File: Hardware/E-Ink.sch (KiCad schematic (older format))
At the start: 4 parts

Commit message: safe commit
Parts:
- removed J?: Micro_USB, digikey-footprints:USB_Micro_B_Female_1050170001, symbol E-Ink:Micro_USB
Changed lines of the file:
@@
 EESchema Schematic File Version 4
-LIBS:E-Ink-cache
 EELAYER 30 0
 EELAYER END
@@
 	1    0    0    -1
 $EndComp
-$Comp
-L E-Ink:Micro_USB J?
-U 1 1 5DC9DD54
-P 4850 2000
-F 0 "J?" H 4914 2723 50  0000 C CNN
-F 1 "Micro_USB" H 4914 2632 50  0000 C CNN
-F 2 "digikey-footprints:USB_Micro_B_Female_1050170001" H 5050 2200 60  0001 L CNN
-F 3 "https://www.molex.com/pdm_docs/sd/1050170001_sd.pdf" H 5050 2300 60  0001 L CNN
-F 4 "WM1399CT-ND" H 5050 2400 60  0001 L CNN "Digi-Key_PN"
-F 5 "1050170001" H 5050 2500 60  0001 L CNN "MPN"
-F 6 "Connectors, Interconnects" H 5050 2600 60  0001 L CNN "Category"
-F 7 "USB, DVI, HDMI Connectors" H 5050 2700 60  0001 L CNN "Family"
-F 8 "https://www.molex.com/pdm_docs/sd/1050170001_sd.pdf" H 5050 2800 60  0001 L CNN "DK_Datasheet_Link"
-F 9 "/product-detail/en/molex/1050170001/WM1399CT-ND/2350885" H 5050 2900 60  0001 L CNN "DK_Detail_Page"
-F 10 "CONN RCPT USB2.0 MICRO B SMD R/A" H 5050 3000 60  0001 L CNN "Description"
-F 11 "Molex" H 5050 3100 60  0001 L CNN "Manufacturer"
-F 12 "Active" H 5050 3200 60  0001 L CNN "Status"
-	1    4850 2000
-	1    0    0    -1
-$EndComp

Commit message: Save commit after work at OTH
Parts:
- removed U?: LDO-3.3V, E-Ink:WSON-6-1EP_3x3mm_P0.95mm, symbol E-Ink:LDO-3.3V
- removed U?: LDO-5.0V, E-Ink:WSON-6-1EP_3x3mm_P0.95mm, symbol E-Ink:LDO-5.0V
- added J?: S8B-PH-SM4-TB, symbol E-Ink:S8B-PH-SM4-TB
- added U?: TXB0104PWR, digikey-footprints:TSSOP-14_W4.4mm, symbol E-Ink:TXB0104PWR
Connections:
- net labels added: +3V3, +5V, BSY_IT8951, CS, EN_SPI, GND, MISO, MOSI, RST_8951, SCK
- wire segments 0 -> 8
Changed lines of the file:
@@
 EESchema Schematic File Version 4
-EELAYER 30 0
+LIBS:E-Ink-cache
+EELAYER 29 0
 EELAYER END
 $Descr A4 11693 8268
@@
 $EndComp
 $Comp
-L E-Ink:LDO-3.3V U?
-U 1 1 5DCA3BF6
-P 4850 3850
-F 0 "U?" H 4925 4555 50  0000 C CNN
-F 1 "LDO-3.3V" H 4925 4464 50  0000 C CNN
-F 2 "E-Ink:WSON-6-1EP_3x3mm_P0.95mm" H 5100 3750 50  0001 C CNN
-F 3 "http://www.ti.com/general/docs/suppproductinfo.tsp?distId=10&gotoUrl=http%3A%2F%2Fwww.ti.com%2Flit%2Fgpn%2Flp38690" H 4700 4450 50  0001 C CNN
-F 4 "LP38692SD-3.3/NOPBCT-ND" H 4925 4373 50  0000 C CNN "Digi-Key_PN"
-	1    4850 3850
+L E-Ink:S8B-PH-SM4-TB J?
+U 1 1 5DD86C25
+P 7100 1500
+F 0 "J?" H 7528 1201 50  0000 L CNN
+F 1 "S8B-PH-SM4-TB" H 7528 1110 50  0000 L CNN
+F 2 "" H 7050 1700 50  0001 C CNN
+F 3 "http://www.jst-mfg.com/product/pdf/eng/ePH.pdf" H 7050 1700 50  0001 C CNN
+F 4 "455-1755-1-ND" H 7450 1600 50  0001 C CNN "Digi-Key_PN"
+	1    7100 1500
 	1    0    0    -1
 $EndComp
 $Comp
-L E-Ink:LDO-5.0V U?
-U 1 1 5DCA47AE
-P 4950 4700
-F 0 "U?" H 4900 5305 50  0000 C CNN
-F 1 "LDO-5.0V" H 4900 5214 50  0000 C CNN
-F 2 "E-Ink:WSON-6-1EP_3x3mm_P0.95mm" H 5000 4500 50  0001 C CNN
-F 3 "http://www.ti.com/general/docs/suppproductinfo.tsp?distId=10&gotoUrl=http%3A%2F%2Fwww.ti.com%2Flit%2Fgpn%2Flp38690" H 4700 5200 50  0001 C CNN
-F 4 "LP38692SD-5.0/NOPBCT-ND" H 4900 5123 50  0000 C CNN "Digi-Key_PN"
-	1    4950 4700
+L power:GND #PWR?
+U 1 1 5DD8AF59
+P 2000 4200
+F 0 "#PWR?" H 2000 3950 50  0001 C CNN
+F 1 "GND" H 2005 4027 50  0000 C CNN
+F 2 "" H 2000 4200 50  0001 C CNN
+F 3 "" H 2000 4200 50  0001 C CNN
+	1    2000 4200
 	1    0    0    -1
 $EndComp
+$Comp
+L power:GND #PWR?
+U 1 1 5DD8BEF7
+P 7100 1600
+F 0 "#PWR?" H 7100 1350 50  0001 C CNN
+F 1 "GND" H 7105 1427 50  0000 C CNN
+F 2 "" H 7100 1600 50  0001 C CNN
+F 3 "" H 7100 1600 50  0001 C CNN
+	1    7100 1600
+	0    1    1    0
+$EndComp
+$Comp
+L power:+5V #PWR?
+U 1 1 5DD8C3B3
+P 7100 1500
+F 0 "#PWR?" H 7100 1350 50  0001 C CNN
+F 1 "+5V" H 7115 1673 50  0000 C CNN
+F 2 "" H 7100 1500 50  0001 C CNN
+F 3 "" H 7100 1500 50  0001 C CNN
+	1    7100 1500
+	1    0    0    -1
+$EndComp
+$Comp
+L power:+5V #PWR?
+U 1 1 5DD8E1F6
+P 4950 1350
+F 0 "#PWR?" H 4950 1200 50  0001 C CNN
+F 1 "+5V" H 4965 1523 50  0000 C CNN
+F 2 "" H 4950 1350 50  0001 C CNN
+F 3 "" H 4950 1350 50  0001 C CNN
+	1    4950 1350
+	1    0    0    -1
+$EndComp
+$Comp
+L power:+3V3 #PWR?
+U 1 1 5DD8E341
+P 4650 1350
+F 0 "#PWR?" H 4650 1200 50  0001 C CNN
+F 1 "+3V3" H 4665 1523 50  0000 C CNN
+F 2 "" H 4650 1350 50  0001 C CNN
+F 3 "" H 4650 1350 50  0001 C CNN
+	1    4650 1350
+	1    0    0    -1
+$EndComp
+Wire Wire Line
+	4650 1350 4750 1350
+Wire Wire Line
+	4750 1350 4750 1400
+Wire Wire Line
+	4850 1400 4850 1350
+Wire Wire Line
+	4850 1350 4950 1350
+$Comp
+L power:GND #PWR?
+U 1 1 5DD8FB9C
+P 4850 2400
+F 0 "#PWR?" H 4850 2150 50  0001 C CNN
+F 1 "GND" H 4855 2227 50  0000 C CNN
+F 2 "" H 4850 2400 50  0001 C CNN
+F 3 "" H 4850 2400 50  0001 C CNN
+	1    4850 2400
+	0    -1   -1   0
+$EndComp
+Wire Wire Line
+	5150 1700 7100 1700
+Wire Wire Line
+	7100 1800 5150 1800
+Wire Wire Line
+	5150 1900 7100 1900
+Wire Wire Line
+	7100 2000 5150 2000
+Text GLabel 4450 1700 0    50   Input ~ 0
+MISO
+Text GLabel 4450 1800 0    50   Input ~ 0
+MOSI
+Text GLabel 4450 1900 0    50   Input ~ 0
+SCK
+Text GLabel 4450 2000 0    50   Input ~ 0
+CS
+Text GLabel 4450 2100 0    50   Input ~ 0
+EN_SPI
+Text GLabel 7100 2100 0    50   Input ~ 0
+RST_8951
+Text GLabel 7100 2200 0    50   Input ~ 0
+BSY_IT8951
+Text GLabel 2600 2200 2    50   Input ~ 0
+MISO
+Text GLabel 2600 2300 2    50   Input ~ 0
+MOSI
+Text GLabel 2600 2400 2    50   Input ~ 0
+SCK
+Text GLabel 2600 2500 2    50   Input ~ 0
+CS
+$Comp
+L E-Ink:TXB0104PWR U?
+U 1 1 5DD8930F
+P 4850 1900
+F 0 "U?" H 4800 1303 60  0000 C CNN
+F 1 "TXB0104PWR" H 4921 1197 60  0000 C CNN
+F 2 "digikey-footprints:TSSOP-14_W4.4mm" H 5050 2100 60  0001 L CNN
+F 3 "http://www.ti.com/general/docs/suppproductinfo.tsp?distId=10&gotoUrl=http%3A%2F%2Fwww.ti.com%2Flit%2Fgpn%2Ftxb0104" H 5050 2200 60  0001 L CNN
+F 4 "296-21929-1-ND" H 5050 2300 60  0001 L CNN "Digi-Key_PN"
+F 5 "TXB0104PWR" H 5050 2400 60  0001 L CNN "MPN"
+F 6 "Integrated Circuits (ICs)" H 5050 2500 60  0001 L CNN "Category"
+F 7 "Logic - Translators, Level Shifters" H 5050 2600 60  0001 L CNN "Family"
+F 8 "http://www.ti.com/general/docs/suppproductinfo.tsp?distId=10&gotoUrl=http%3A%2F%2Fwww.ti.com%2Flit%2Fgpn%2Ftxb0104" H 5050 2700 60  0001 L CNN "DK_Datasheet_Link"
+F 9 "/product-detail/en/texas-instruments/TXB0104PWR/296-21929-1-ND/1629282" H 5050 2800 60  0001 L CNN "DK_Detail_Page"
+F 10 "IC TRNSLTR BIDIRECTIONAL 14TSSOP" H 5050 2900 60  0001 L CNN "Description"
+F 11 "Texas Instruments" H 5050 3000 60  0001 L CNN "Manufacturer"
+F 12 "Active" H 5050 3100 60  0001 L CNN "Status"
+	1    4850 1900
+	1    0    0    -1
+$EndComp

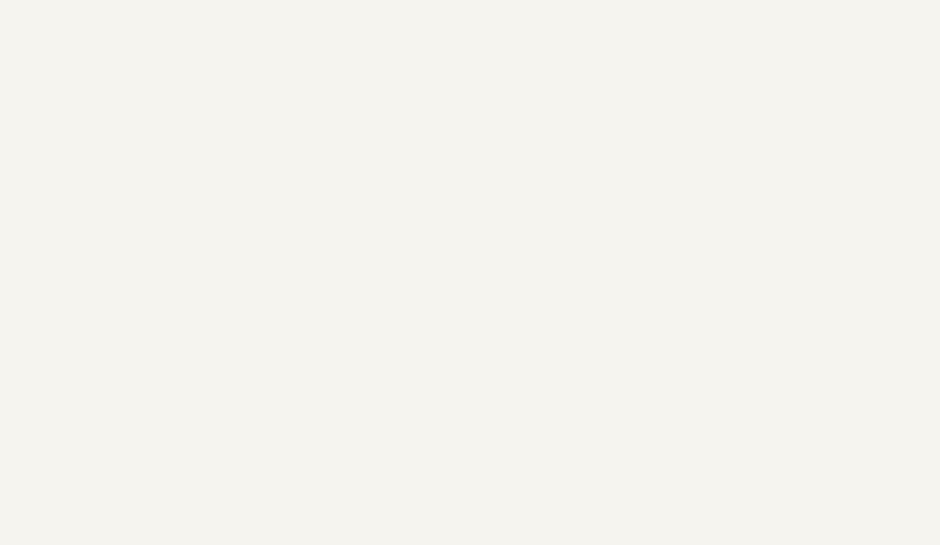
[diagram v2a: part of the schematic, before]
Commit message: save work at oth
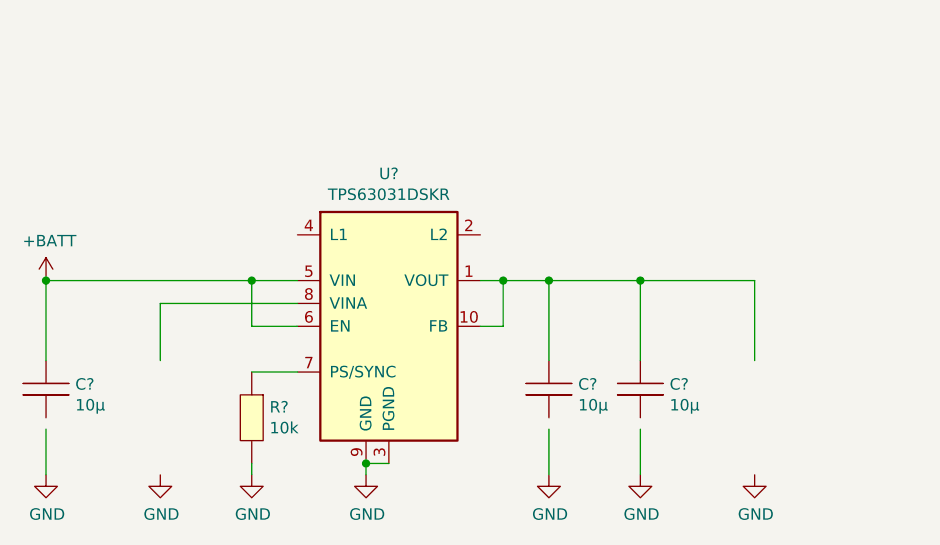
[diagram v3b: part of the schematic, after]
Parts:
- added C? (x3): 10µ, Capacitor_SMD:C_0805_2012Metric_Pad1.15x1.40mm_HandSolder, symbol E-Ink:10µ
- added R?: 10k, Resistor_SMD:R_0805_2012Metric_Pad1.15x1.40mm_HandSolder, symbol E-Ink:10k
- added U?: TPS63031DSKR, Package_SON:Texas_S-PWSON-N10, symbol E-Ink:TPS63031DSKR
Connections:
- net labels added: +BATT
- wire segments 8 -> 31
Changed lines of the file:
@@
 	1    0    0    -1
 $EndComp
+$Comp
+L E-Ink:TPS63031DSKR U?
+U 1 1 5DDC1A9A
+P 2000 5900
+F 0 "U?" H 2300 5967 50  0000 C CNN
+F 1 "TPS63031DSKR" H 2300 5876 50  0000 C CNN
+F 2 "Package_SON:Texas_S-PWSON-N10" H 2700 5950 50  0001 C CNN
+F 3 "http://www.ti.com/general/docs/suppproductinfo.tsp?distId=10&gotoUrl=http%3A%2F%2Fwww.ti.com%2Flit%2Fgpn%2Ftps63030" H 2050 5850 50  0001 C CNN
+F 4 "296-39461-1-ND" H 2400 6050 50  0001 C CNN "Digi-Key_PN"
+	1    2000 5900
+	1    0    0    -1
+$EndComp
+$Comp
+L power:+BATT #PWR?
+U 1 1 5DDC2D4D
+P 800 6300
+F 0 "#PWR?" H 800 6150 50  0001 C CNN
+F 1 "+BATT" H 815 6473 50  0000 C CNN
+F 2 "" H 800 6300 50  0001 C CNN
+F 3 "" H 800 6300 50  0001 C CNN
+	1    800  6300
+	1    0    0    -1
+$EndComp
+$Comp
+L power:GND #PWR?
+U 1 1 5DDC409F
+P 2200 7150
+F 0 "#PWR?" H 2200 6900 50  0001 C CNN
+F 1 "GND" H 2205 6977 50  0000 C CNN
+F 2 "" H 2200 7150 50  0001 C CNN
+F 3 "" H 2200 7150 50  0001 C CNN
+	1    2200 7150
+	1    0    0    -1
+$EndComp
+Wire Wire Line
+	2200 7100 2200 7150
+Wire Wire Line
+	2200 7100 2300 7100
+Connection ~ 2200 7100
+Wire Wire Line
+	1900 6300 1700 6300
+Wire Wire Line
+	1900 6500 1700 6500
+Wire Wire Line
+	1700 6500 1700 6300
+Connection ~ 1700 6300
+Wire Wire Line
+	1700 6300 800  6300
+$Comp
+L E-Ink:10k R?
+U 1 1 5DDC55C2
+P 1750 6800
+F 0 "R?" V 1804 6828 50  0000 L CNN
+F 1 "10k" V 1895 6828 50  0000 L CNN
+F 2 "Resistor_SMD:R_0805_2012Metric_Pad1.15x1.40mm_HandSolder" H 1800 6650 50  0001 C CNN
+F 3 "" H 1750 6850 50  0001 C CNN
+	1    1750 6800
+	0    1    1    0
+$EndComp
+Wire Wire Line
+	1700 6700 1900 6700
+$Comp
+L power:GND #PWR?
+U 1 1 5DDC6FD7
+P 1700 7150
+F 0 "#PWR?" H 1700 6900 50  0001 C CNN
+F 1 "GND" H 1705 6977 50  0000 C CNN
+F 2 "" H 1700 7150 50  0001 C CNN
+F 3 "" H 1700 7150 50  0001 C CNN
+	1    1700 7150
+	1    0    0    -1
+$EndComp
+Wire Wire Line
+	1700 7100 1700 7150
+$Comp
+L power:GND #PWR?
+U 1 1 5DDC7D0E
+P 1300 7150
+F 0 "#PWR?" H 1300 6900 50  0001 C CNN
+F 1 "GND" H 1305 6977 50  0000 C CNN
+F 2 "" H 1300 7150 50  0001 C CNN
+F 3 "" H 1300 7150 50  0001 C CNN
+	1    1300 7150
+	1    0    0    -1
+$EndComp
+$Comp
+L power:GND #PWR?
+U 1 1 5DDC7EFC
+P 800 7150
+F 0 "#PWR?" H 800 6900 50  0001 C CNN
+F 1 "GND" H 805 6977 50  0000 C CNN
+F 2 "" H 800 7150 50  0001 C CNN
+F 3 "" H 800 7150 50  0001 C CNN
+	1    800  7150
+	1    0    0    -1
+$EndComp
+$Comp
+L E-Ink:10µ C?
+U 1 1 5DDC8130
+P 950 6800
+F 0 "C?" V 904 6778 50  0000 L CNN
+F 1 "10µ" V 995 6778 50  0000 L CNN
+F 2 "Capacitor_SMD:C_0805_2012Metric_Pad1.15x1.40mm_HandSolder" H 950 6500 50  0001 C CNN
+F 3 "" H 900 6800 50  0001 C CNN
+	1    950  6800
+	0    1    1    0
+$EndComp
+Wire Wire Line
+	1300 6650 1300 6400
+Wire Wire Line
+	1300 6400 1900 6400
+Connection ~ 800  6300
+Wire Wire Line
+	800  6300 800  6650
+Wire Wire Line
+	800  6950 800  7150
+Wire Wire Line
+	2700 6500 2800 6500
+Wire Wire Line
+	2800 6500 2800 6300
+Wire Wire Line
+	2800 6300 2700 6300
+$Comp
+L E-Ink:10µ C?
+U 1 1 5DDCE133
+P 3550 6800
+F 0 "C?" V 3504 6778 50  0000 L CNN
+F 1 "10µ" V 3595 6778 50  0000 L CNN
+F 2 "Capacitor_SMD:C_0805_2012Metric_Pad1.15x1.40mm_HandSolder" H 3550 6500 50  0001 C CNN
+F 3 "" H 3500 6800 50  0001 C CNN
+	1    3550 6800
+	0    1    1    0
+$EndComp
+Wire Wire Line
+	3400 6300 3400 6650
+$Comp
+L E-Ink:10µ C?
+U 1 1 5DDCE670
+P 3150 6800
+F 0 "C?" V 3104 6778 50  0000 L CNN
+F 1 "10µ" V 3195 6778 50  0000 L CNN
+F 2 "Capacitor_SMD:C_0805_2012Metric_Pad1.15x1.40mm_HandSolder" H 3150 6500 50  0001 C CNN
+F 3 "" H 3100 6800 50  0001 C CNN
+	1    3150 6800
+	0    1    1    0
+$EndComp
+Wire Wire Line
+	2800 6300 3000 6300
+Connection ~ 2800 6300
+Wire Wire Line
+	3900 6300 3400 6300
+Wire Wire Line
+	3900 6300 3900 6650
+Connection ~ 3400 6300
+Connection ~ 3000 6300
+Wire Wire Line
+	3000 6300 3400 6300
+Wire Wire Line
+	3000 6300 3000 6650
+$Comp
+L power:GND #PWR?
+U 1 1 5DDD090A
+P 3900 7150
+F 0 "#PWR?" H 3900 6900 50  0001 C CNN
+F 1 "GND" H 3905 6977 50  0000 C CNN
+F 2 "" H 3900 7150 50  0001 C CNN
+F 3 "" H 3900 7150 50  0001 C CNN
+	1    3900 7150
+	1    0    0    -1
+$EndComp
+$Comp
+L power:GND #PWR?
+U 1 1 5DDD0910
+P 3400 7150
+F 0 "#PWR?" H 3400 6900 50  0001 C CNN
+F 1 "GND" H 3405 6977 50  0000 C CNN
+F 2 "" H 3400 7150 50  0001 C CNN
+F 3 "" H 3400 7150 50  0001 C CNN
+	1    3400 7150
+	1    0    0    -1
+$EndComp
+$Comp
+L power:GND #PWR?
+U 1 1 5DDD0916
+P 3000 7150
+F 0 "#PWR?" H 3000 6900 50  0001 C CNN
+F 1 "GND" H 3005 6977 50  0000 C CNN
+F 2 "" H 3000 7150 50  0001 C CNN
+F 3 "" H 3000 7150 50  0001 C CNN
+	1    3000 7150
+	1    0    0    -1
+$EndComp
+Wire Wire Line
+	3000 6950 3000 7150
+Wire Wire Line
+	3400 6950 3400 7150
 $EndSCHEMATC

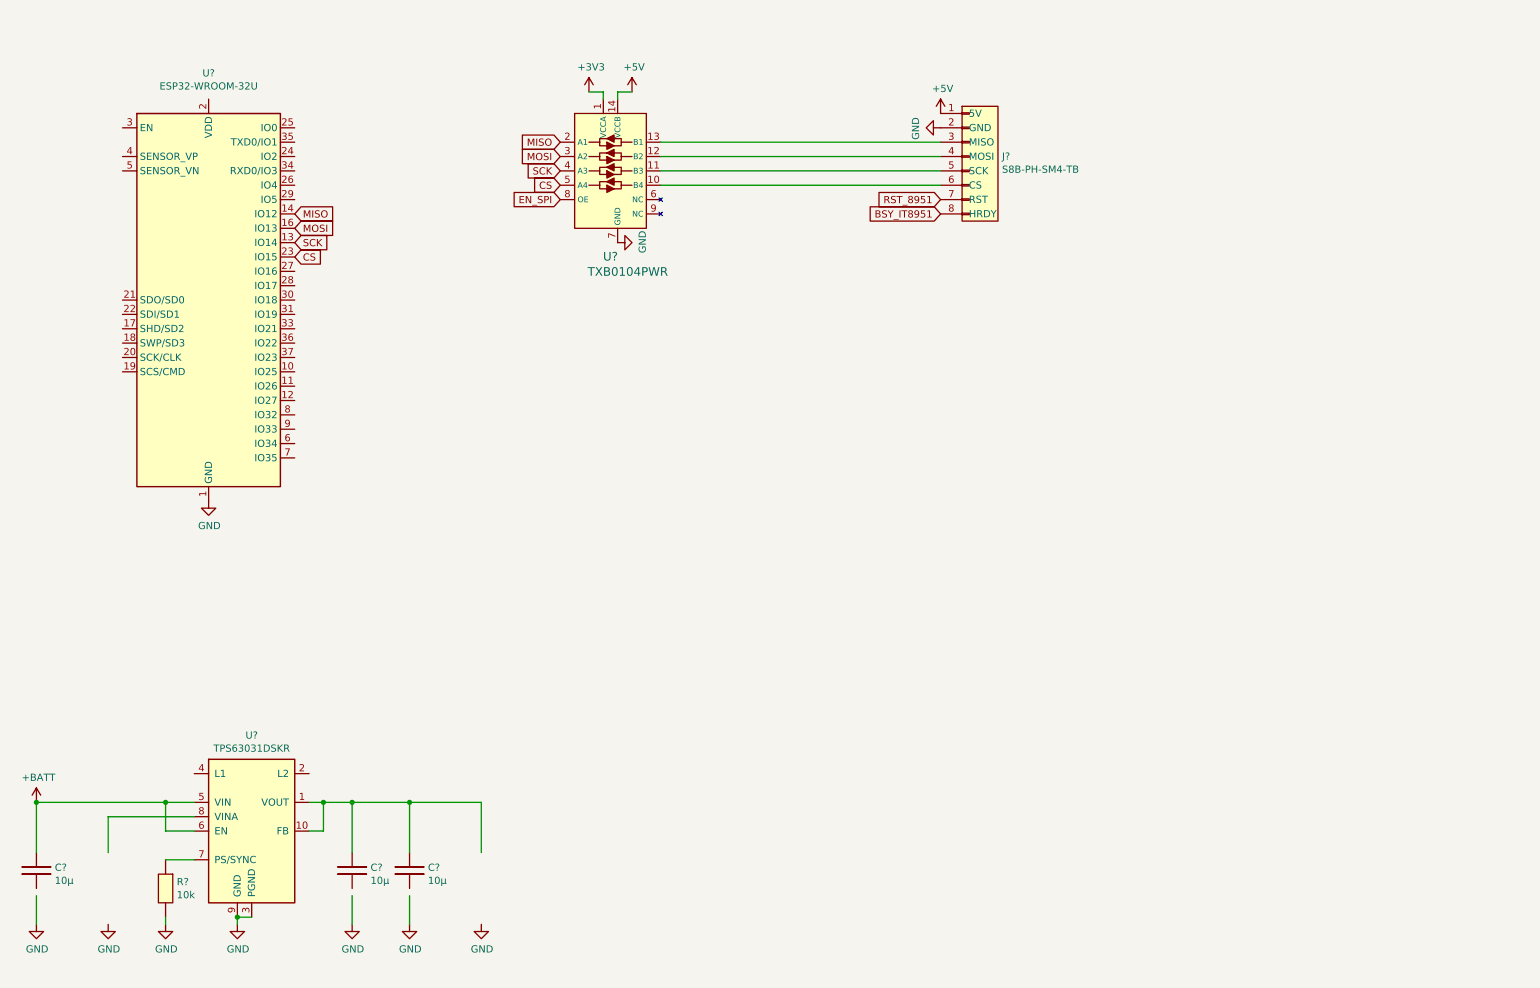
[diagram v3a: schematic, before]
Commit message: save commit again
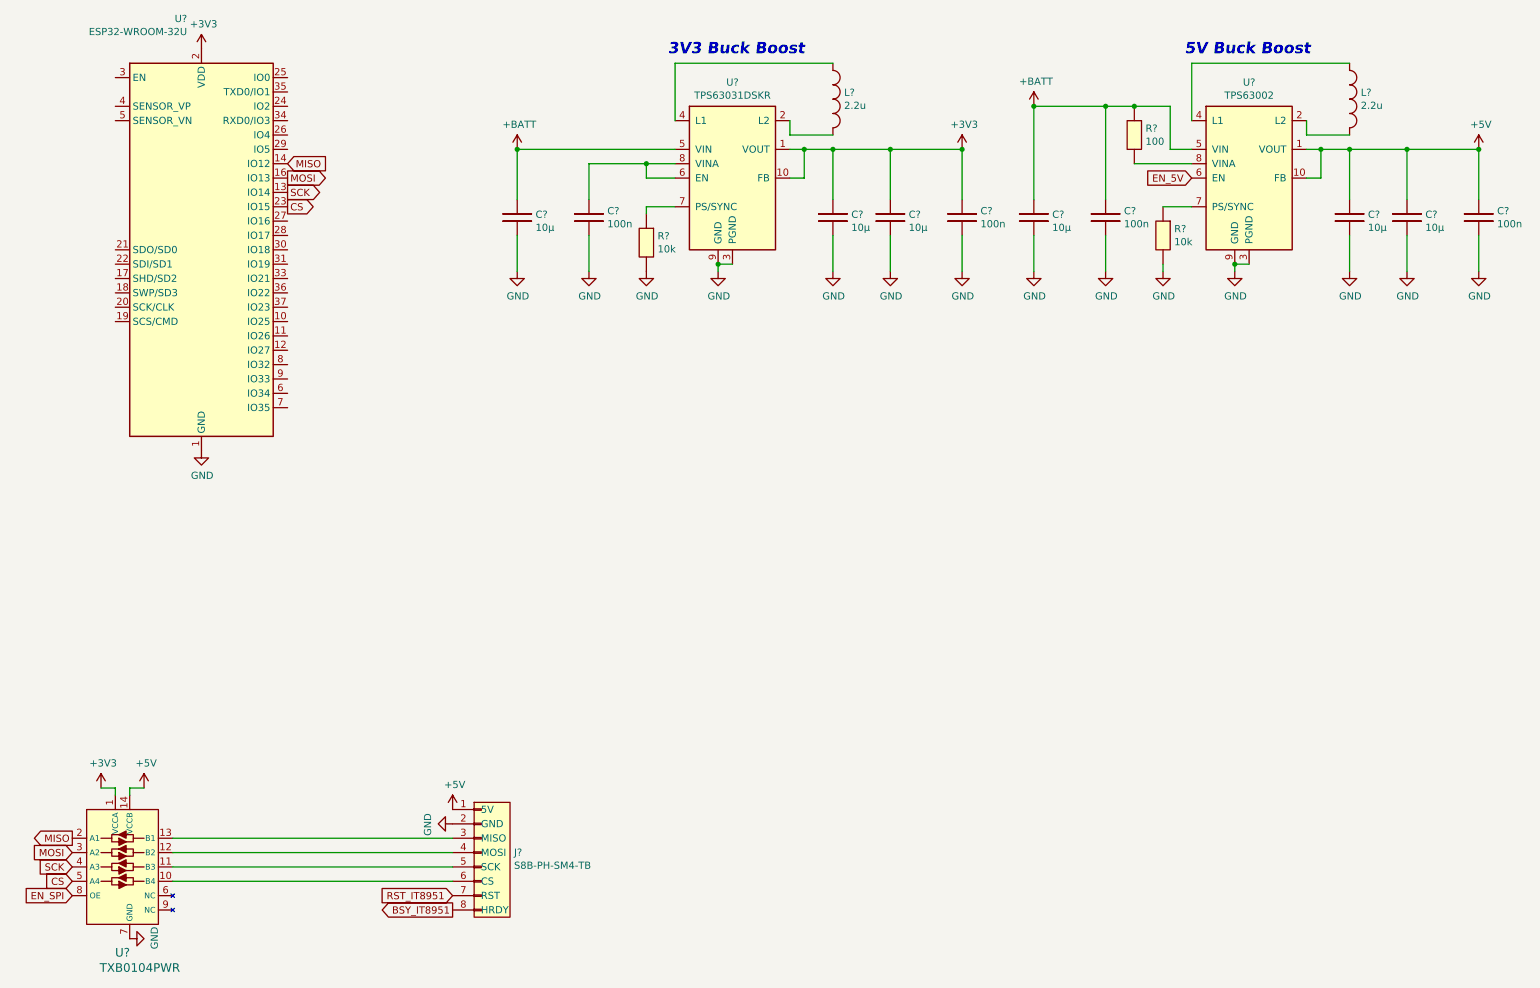
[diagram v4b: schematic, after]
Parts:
- removed R?: 10k, Resistor_SMD:R_0805_2012Metric_Pad1.15x1.40mm_HandSolder, symbol E-Ink:10k
- added C? (x4): 100n, Capacitor_SMD:C_0805_2012Metric_Pad1.15x1.40mm_HandSolder, symbol E-Ink:100n
- added C? (x3): 10µ, Capacitor_SMD:C_0805_2012Metric_Pad1.15x1.40mm_HandSolder, symbol E-Ink:10µ
- added L? (x2): 2.2u, symbol E-Ink:2.2u
- added R? (x2): 10k, Resistor_SMD:R_0805_2012Metric_Pad1.15x1.40mm_HandSolder, symbol E-Ink:10k
- added R?: 100, Resistor_SMD:R_0805_2012Metric_Pad1.15x1.40mm_HandSolder, symbol E-Ink:100
- added U?: TPS63002, Package_SON:Texas_DRC0010J_ThermalVias, symbol E-Ink:TPS63002DRCR
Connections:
- net labels added: EN_5V, RST_IT8951
- net labels removed: RST_8951
- wire segments 31 -> 67
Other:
- note added: "3V3 Buck Boost"
- note added: "5V Buck Boost"
- moved on the sheet: C?, J?, U?
